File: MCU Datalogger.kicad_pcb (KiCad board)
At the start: 2 copper layers, 43 x 36.2 mm, 29 parts, among them J1 Conn_01x04_Pin, J2 Conn_01x04_Pin, J3 Conn_01x09_Pin, J4 Conn_02x03_Odd_Even, U1 24LC1025, U2 24LC1025, U3 DS1337S_, U4 ATMEGA328P-AU, Y1 32.768 KHz, Y2 16 MHz

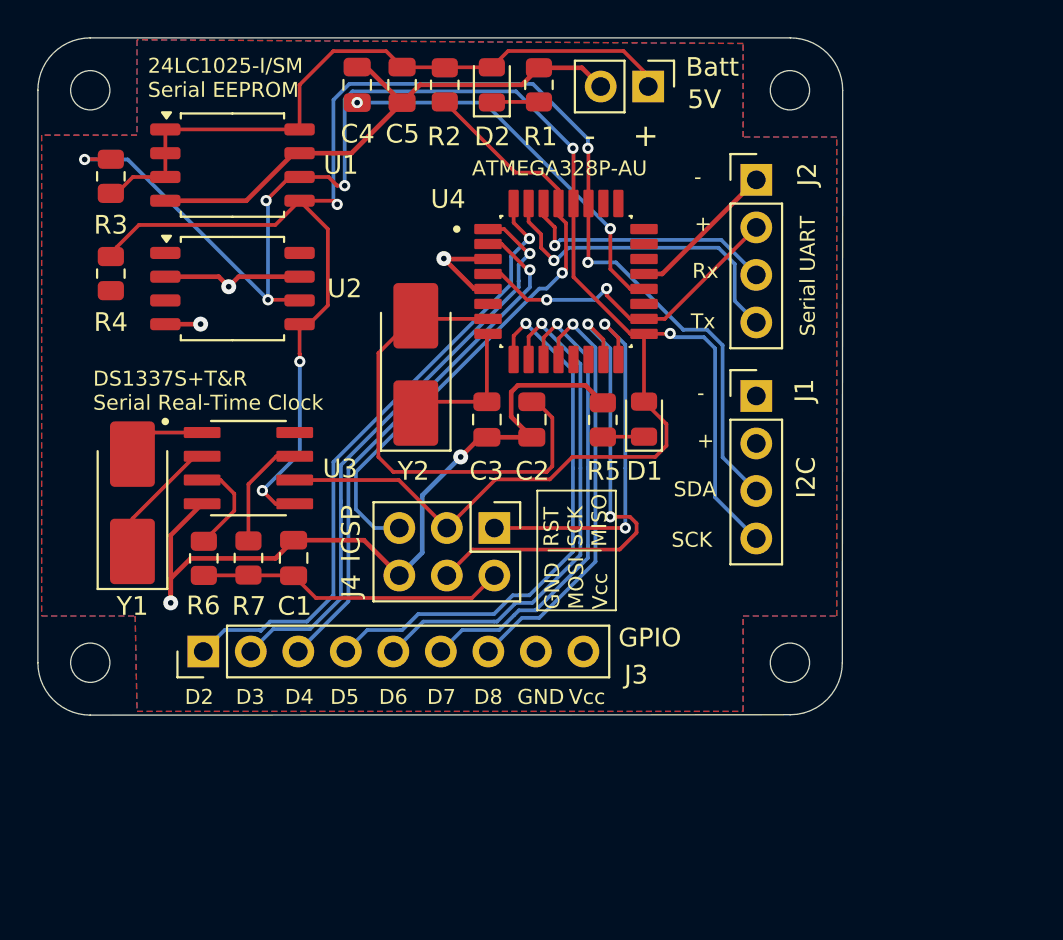
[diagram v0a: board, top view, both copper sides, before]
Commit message: Updates
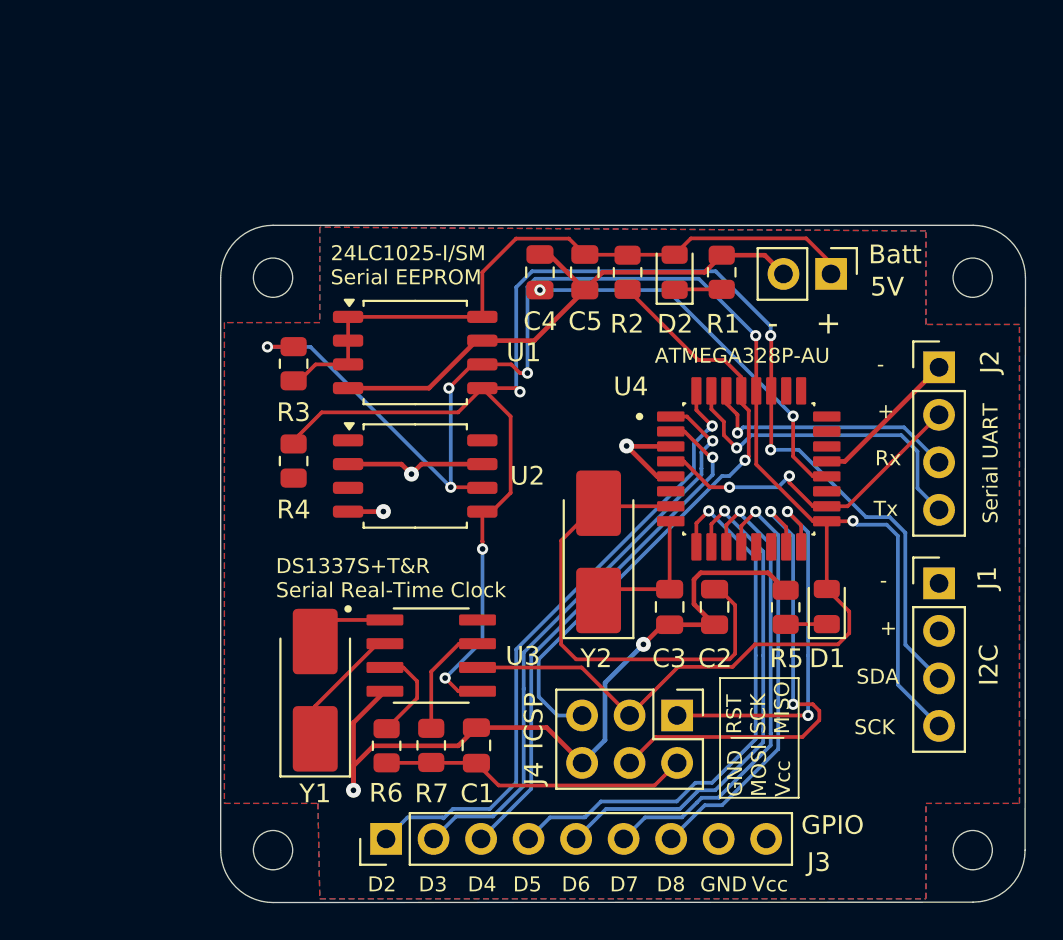
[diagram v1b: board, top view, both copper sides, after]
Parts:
- moved J3 14.0 mm to (133.2, 116.6)
- moved U1 14.0 mm to (134.8, 90.6)
- moved BT1 14.0 mm to (157.0, 86.4)
- moved C2 14.0 mm to (150.8, 104.2)
- moved C3 14.0 mm to (148.4, 104.2)
- moved C4 14.0 mm to (141.4, 86.3)
- moved C5 14.0 mm to (143.8, 86.3)
- moved D1 14.0 mm to (156.8, 104.2)
- moved H1 14.0 mm to (127.2, 86.6)
- moved J1 14.0 mm to (162.8, 103.0)
- moved J2 14.0 mm to (162.8, 91.4)
- moved J4 14.0 mm to (148.8, 110.0)
- moved R1 14.0 mm to (151.2, 86.3)
- moved R2 14.0 mm to (146.1, 86.3)
- moved R3 14.0 mm to (128.3, 91.2)
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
